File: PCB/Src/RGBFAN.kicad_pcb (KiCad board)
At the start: 2 copper layers, 104.1 x 66 mm, 13 parts

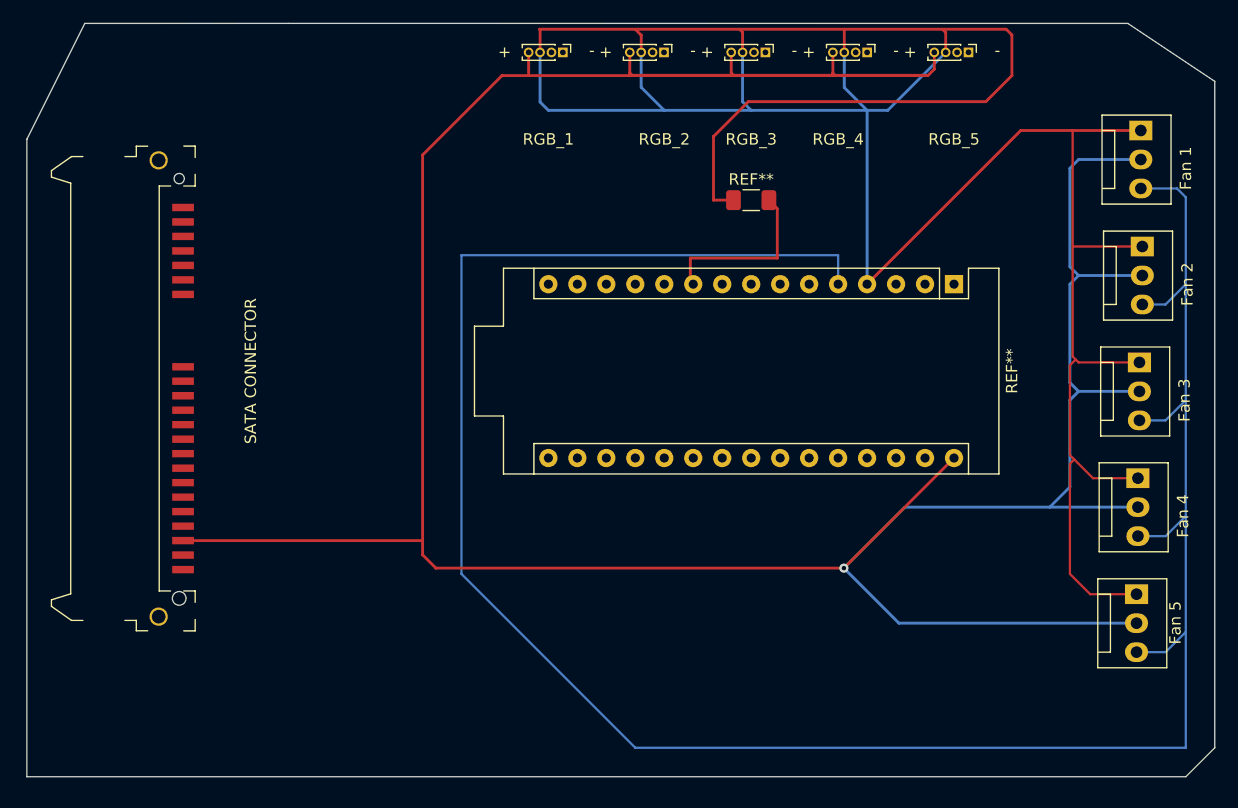
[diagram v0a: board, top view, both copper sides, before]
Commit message: more changes
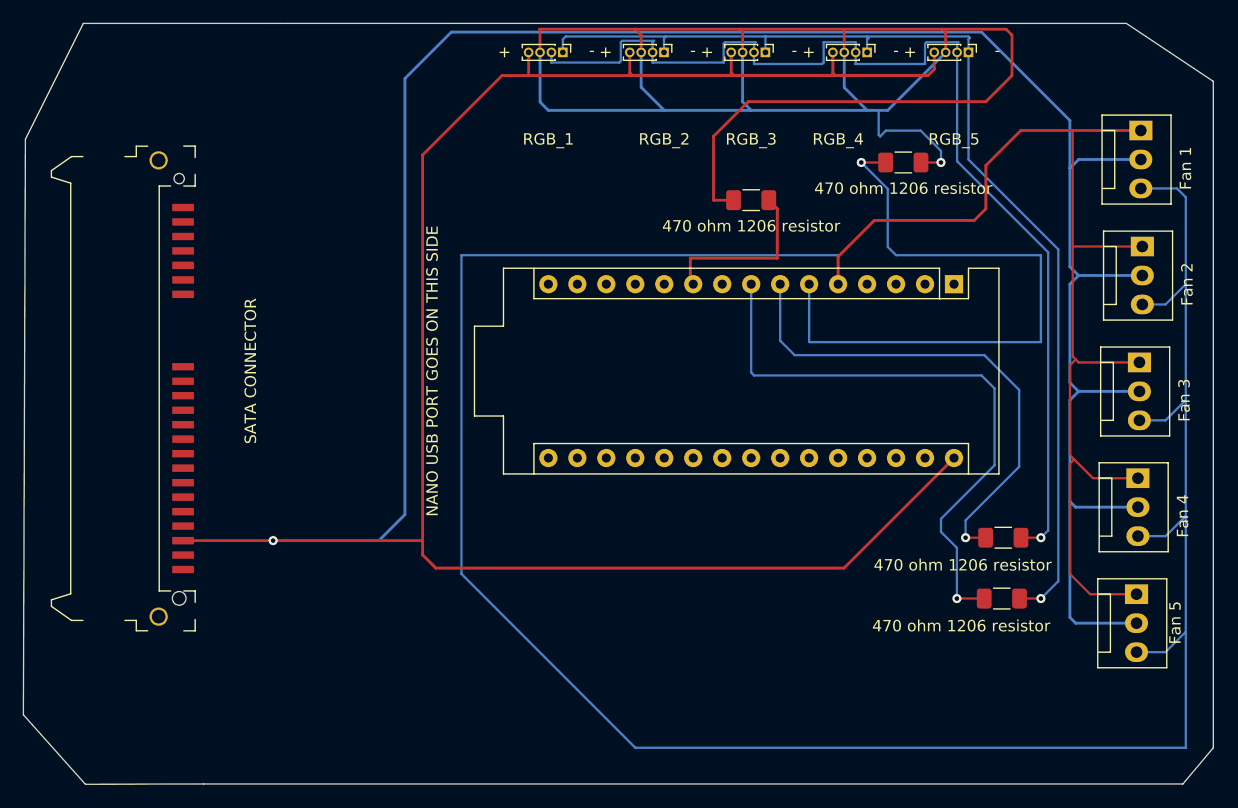
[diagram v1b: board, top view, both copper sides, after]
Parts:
- added 470 ohm 1206 resistor: R_1206_3216Metric_Pad1.30x1.75mm_HandSolder, Resistor_SMD:R_1206_3216Metric_Pad1.30x1.75mm_HandSolder, F.Cu at (151.5, 113.9)
- added 470 ohm 1206 resistor: R_1206_3216Metric_Pad1.30x1.75mm_HandSolder, Resistor_SMD:R_1206_3216Metric_Pad1.30x1.75mm_HandSolder, F.Cu at (151.6, 108.6)
- added 470 ohm 1206 resistor: R_1206_3216Metric_Pad1.30x1.75mm_HandSolder, Resistor_SMD:R_1206_3216Metric_Pad1.30x1.75mm_HandSolder, F.Cu at (142.9, 75.7)
- 470 ohm 1206 resistor: renamed from REF**
- NANO USB PORT GOES ON THIS SIDE: renamed from REF**
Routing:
- net (no net): track 775.9 -> 1211.7 mm, vias 1 -> 7
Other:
- board size 104.1 x 66 mm -> 104.3 x 66.7 mm
